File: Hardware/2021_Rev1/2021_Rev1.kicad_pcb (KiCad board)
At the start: 2 copper layers, 124.5 x 81.3 mm, 49 parts, among them J1 USB_A, U1 TM4C129E_Launchpad, U2 OKI, U3 OKI, U4 FT230XS

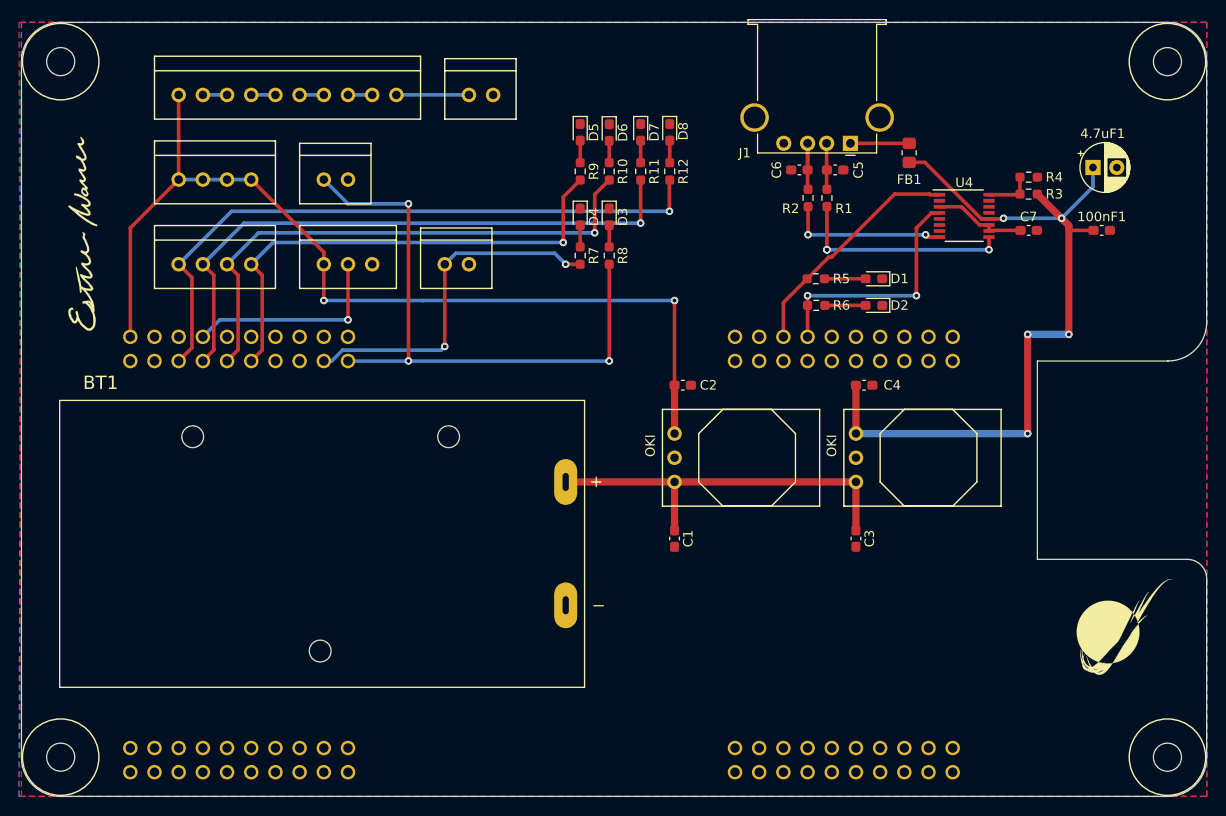
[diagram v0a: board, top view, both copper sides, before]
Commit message: tiva footprint changed to THT_BOTTOM
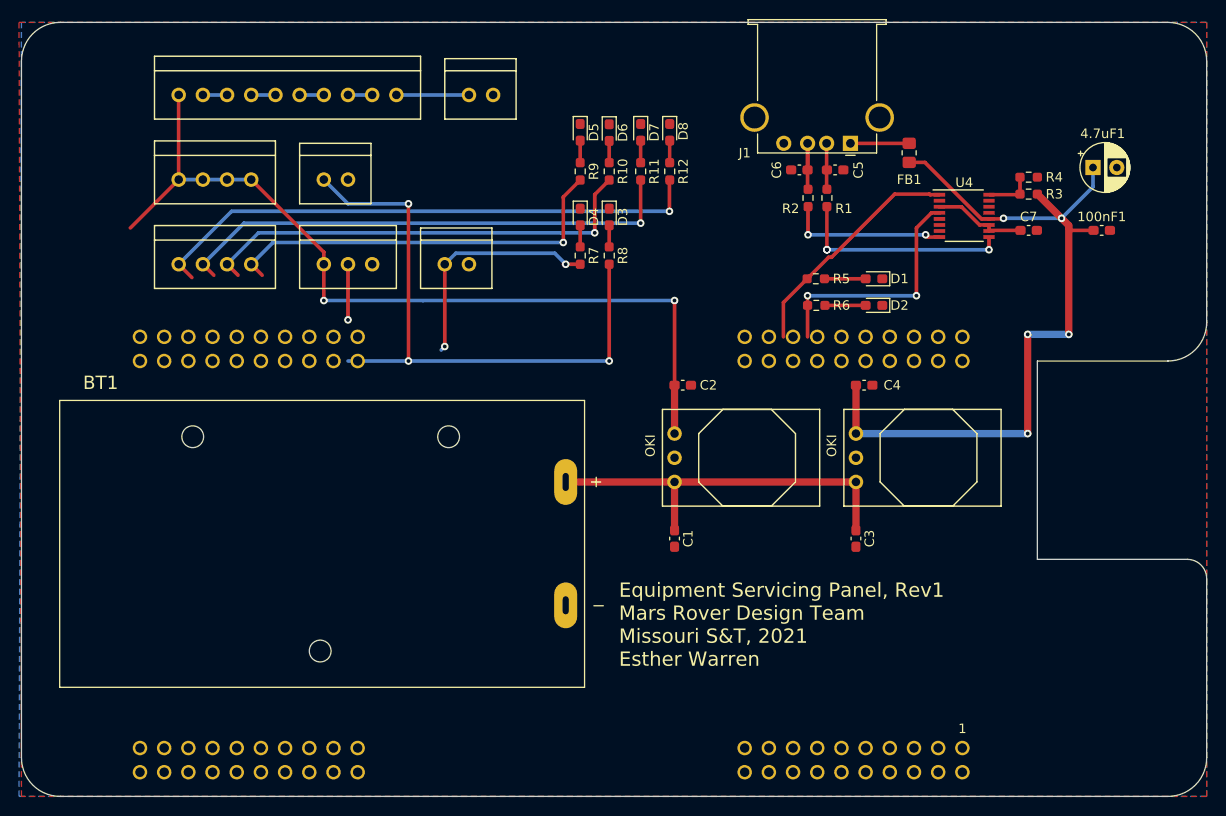
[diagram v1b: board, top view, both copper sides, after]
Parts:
- removed G***: LOGO, MRDT_Silkscreens:0_MRDT_Logo_10mm
- removed G***: LOGO, Packages:Signature_15mm_Esther
- removed REF** (x4): 4_40_Hole, MRDT_Drill_Holes:4_40_Hole_Corner
- U1: footprint MRDT_Shields:TM4C129E_Launchpad_FULL_THT_TOP -> MRDT_Shields:TM4C129E_Launchpad_FULL_THT_BOTTOM; moved to F.Cu
- moved U1 89.9 mm to (996.7, -213.4), turned to 180 degrees
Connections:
- J1 pad 5: GND -> Net-(J1-Pad5)
- J1 pad e5: GND -> (no net)
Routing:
- net LCD_TX: track 21.8 -> 5.84 mm
- net AZI_CTL: track 37.4 -> 24.6 mm
- net +3V3: track 101.8 -> 90.4 mm
- net ELEV_MINUS: track 63.4 -> 53.9 mm
- net AZI_PLUS: track 57.3 -> 47.8 mm
- net AZI_MINUS: track 52.1 -> 42.6 mm
- net ELEV_PLUS: track 68.4 -> 59.1 mm
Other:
- board text added: "Equipment Servicing Panel, Rev1 Mars Rover Design Team Missouri S&T, 2021 Esther Warren"

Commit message: Revert "tiva footprint changed to THT_BOTTOM"
This reverts commit b87381c65a80fcd5fad75ae35fe4b21bdfbb7d2f.
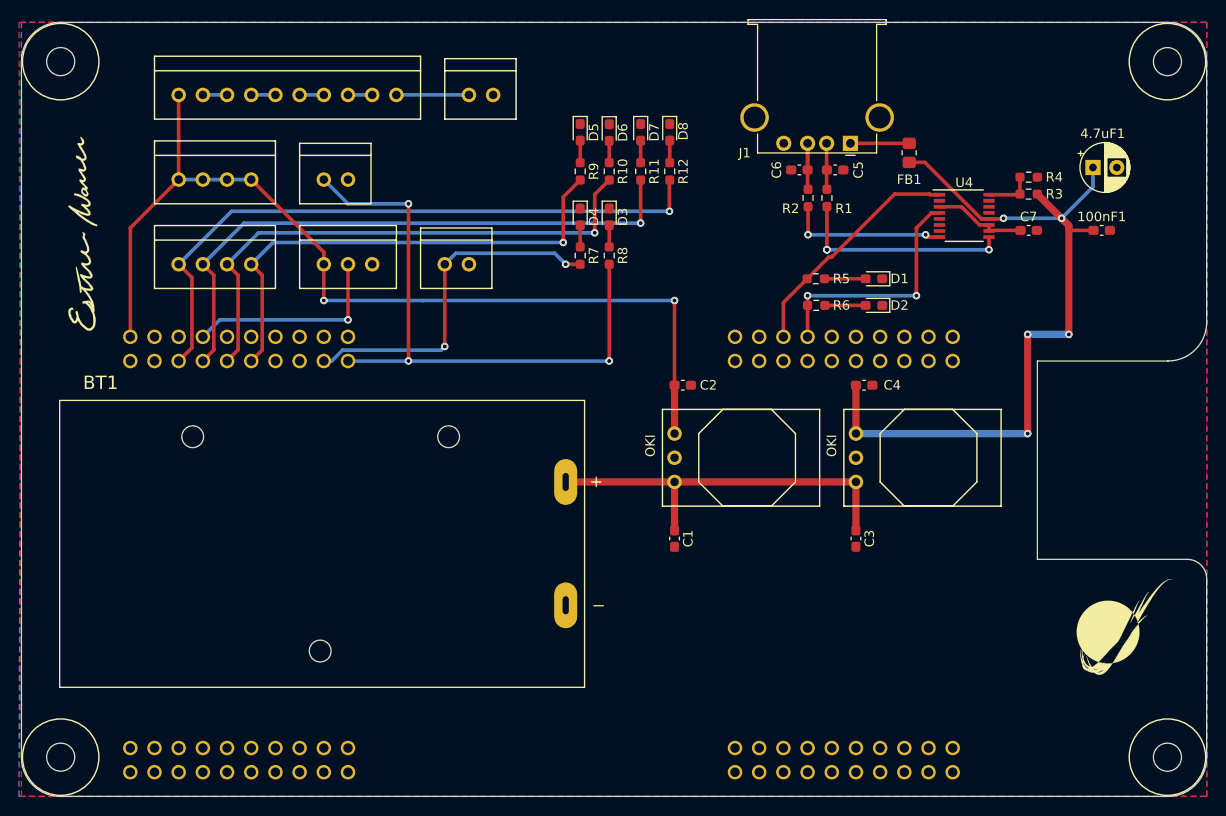
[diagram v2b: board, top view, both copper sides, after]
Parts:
- added G***: LOGO, MRDT_Silkscreens:0_MRDT_Logo_10mm, F.Cu at (1012.4, -181.6)
- added G***: LOGO, Packages:Signature_15mm_Esther, F.Cu at (902.5, -220.5)
- added REF**: 4_40_Hole, MRDT_Drill_Holes:4_40_Hole_Corner, F.Cu at (1013.0, -237.0)
- added REF**: 4_40_Hole, MRDT_Drill_Holes:4_40_Hole_Corner, F.Cu at (1013.0, -172.0)
- added REF**: 4_40_Hole, MRDT_Drill_Holes:4_40_Hole_Corner, F.Cu at (904.7, -172.0)
- added REF**: 4_40_Hole, MRDT_Drill_Holes:4_40_Hole_Corner, F.Cu at (904.7, -237.0)
- U1: footprint MRDT_Shields:TM4C129E_Launchpad_FULL_THT_BOTTOM -> MRDT_Shields:TM4C129E_Launchpad_FULL_THT_TOP; moved to B.Cu
- moved U1 89.9 mm to (906.8, -213.4), turned to 0 degrees
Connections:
- J1 pad 5: Net-(J1-Pad5) -> GND
- J1 pad e5: (no net) -> GND
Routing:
- net LCD_TX: track 5.84 -> 21.8 mm
- net AZI_CTL: track 24.6 -> 37.4 mm
- net +3V3: track 90.4 -> 101.8 mm
- net ELEV_MINUS: track 53.9 -> 63.4 mm
- net AZI_PLUS: track 47.8 -> 57.3 mm
- net AZI_MINUS: track 42.6 -> 52.1 mm
- net ELEV_PLUS: track 59.1 -> 68.4 mm
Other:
- board text removed: "Equipment Servicing Panel, Rev1 Mars Rover Design Team Missouri S&T, 2021 Esther Warren"
